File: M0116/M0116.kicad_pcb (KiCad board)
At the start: 2 copper layers, 38 x 17 mm, 2 parts, among them J2 Conn_01x04

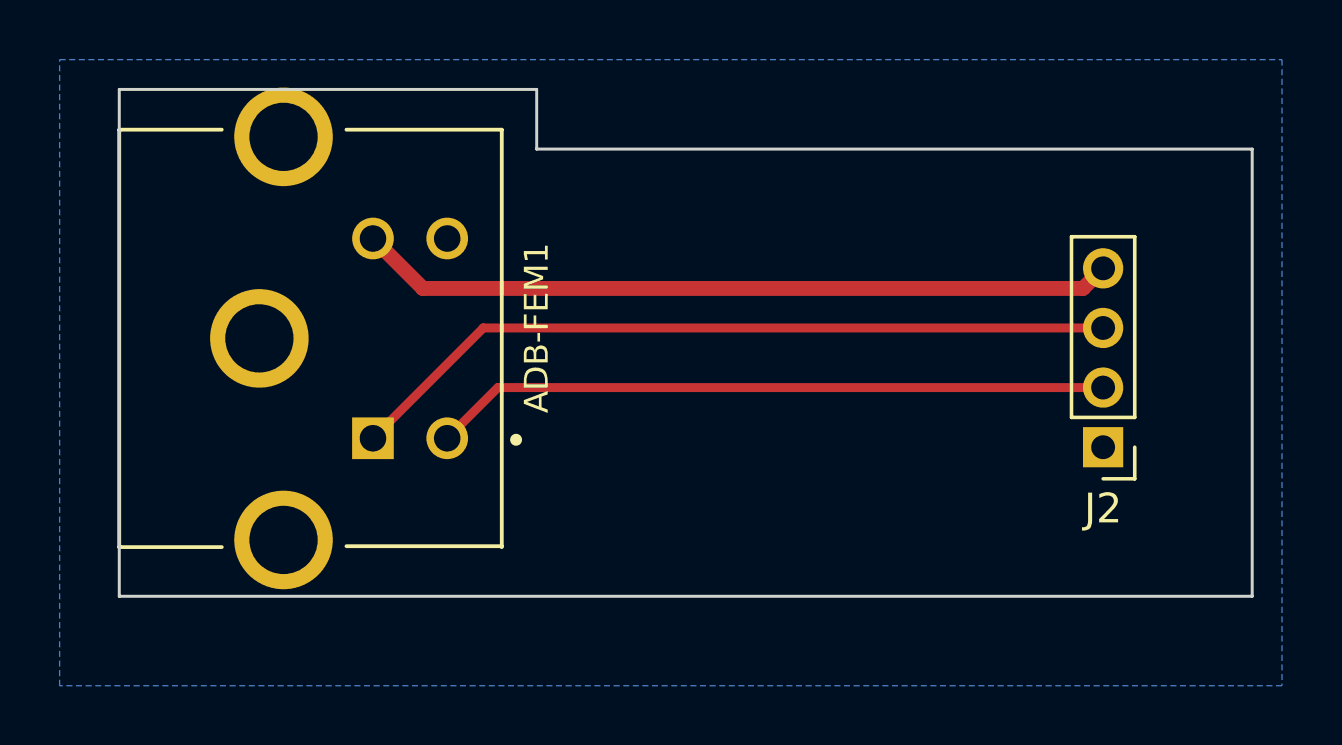
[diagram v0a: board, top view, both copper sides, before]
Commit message: added fabrication outputs
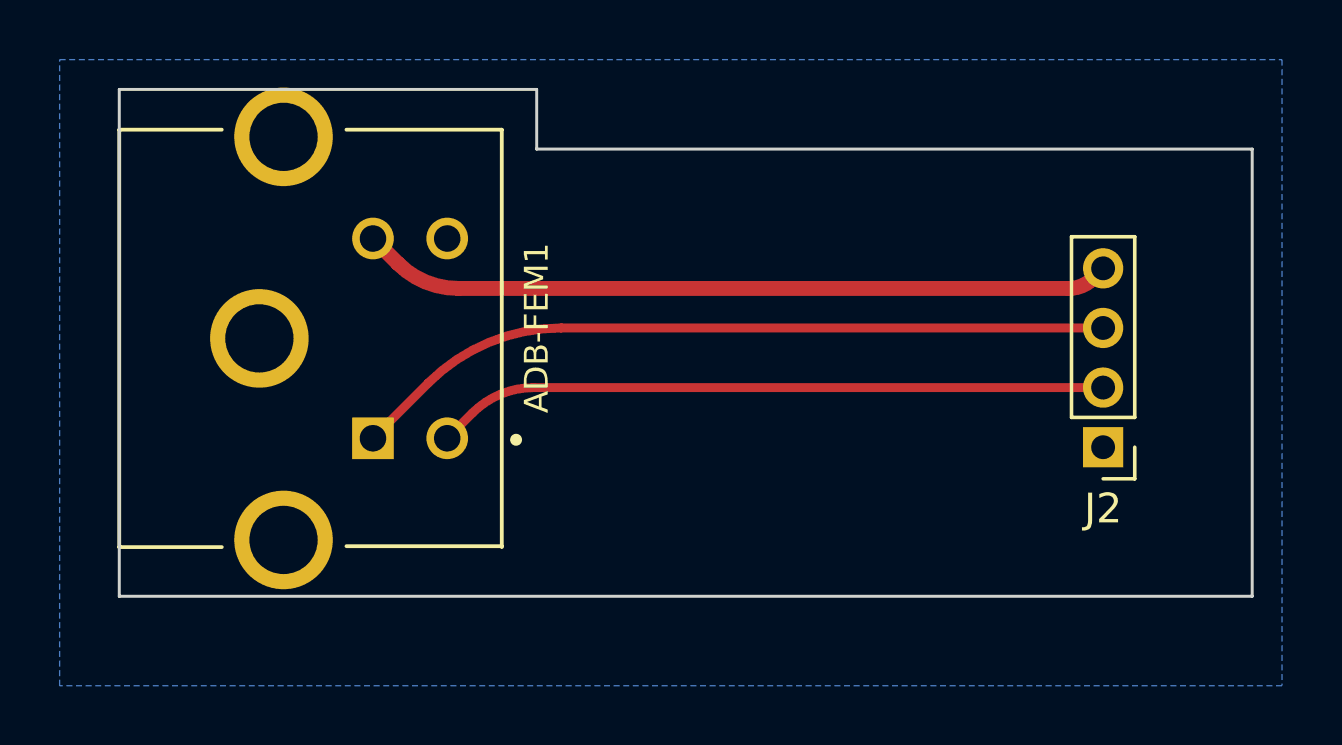
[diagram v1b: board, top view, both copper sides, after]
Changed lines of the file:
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@@
   (gr_line (start 114 102) (end 114 100)
     (stroke (width 0.1) (type default)) (layer "Edge.Cuts"))
-  (segment (start 133 108) (end 112.21 108) (width 0.3) (layer "F.Cu") (net 1))
-  (segment (start 112.21 108) (end 108.51 111.7) (width 0.3) (layer "F.Cu") (net 1))
-  (segment (start 112.7 110) (end 111 111.7) (width 0.3) (layer "F.Cu") (net 2))
-  (segment (start 133 110) (end 112.7 110) (width 0.3) (layer "F.Cu") (net 2))
-  (segment (start 133 106) (end 132.325 106.675) (width 0.5) (layer "F.Cu") (net 3))
-  (segment (start 110.185 106.675) (end 108.51 105) (width 0.5) (layer "F.Cu") (net 3))
-  (segment (start 132.325 106.675) (end 110.185 106.675) (width 0.5) (layer "F.Cu") (net 3))
+  (segment (start 114.826295 108) (end 133 108) (width 0.3) (layer "F.Cu") (net 1))
+  (segment (start 110.36 109.85) (end 108.51 111.7) (width 0.3) (layer "F.Cu") (net 1))
+  (arc (start 114.826295 108) (mid 112.409153 108.480799) (end 110.36 109.85) (width 0.3) (layer "F.Cu") (net 1))
+  (segment (start 111.85 110.85) (end 111 111.7) (width 0.3) (layer "F.Cu") (net 2))
+  (segment (start 113.902081 110) (end 133 110) (width 0.3) (layer "F.Cu") (net 2))
+  (arc (start 113.902081 110) (mid 112.791502 110.220907) (end 111.85 110.85) (width 0.3) (layer "F.Cu") (net 2))
+  (segment (start 132.6625 106.3375) (end 133 106) (width 0.5) (layer "F.Cu") (net 3))
+  (segment (start 109.3475 105.8375) (end 108.51 105) (width 0.5) (layer "F.Cu") (net 3))
+  (segment (start 111.369403 106.675) (end 131.847702 106.675) (width 0.5) (layer "F.Cu") (net 3))
+  (arc (start 132.6625 106.3375) (mid 132.288667 106.587286) (end 131.847702 106.675) (width 0.5) (layer "F.Cu") (net 3))
+  (arc (start 109.3475 105.8375) (mid 110.275157 106.45734) (end 111.369403 106.675) (width 0.5) (layer "F.Cu") (net 3))
+  (zone (net 2) (net_name "JST-D-") (layer "F.Cu") (name "$teardrop_padvia$") (hatch edge 0.5)
+    (priority 30004)
+    (attr (teardrop (type padvia)))
+    (connect_pads yes (clearance 0))
+    (min_thickness 0.0254) (filled_areas_thickness no)
+    (fill yes (thermal_gap 0.5) (thermal_bridge_width 0.5) (island_removal_mode 1) (island_area_min 10))
+    (polygon
+      (pts
+        (xy 131.65 109.85)
+        (xy 131.65 110.15)
+        (xy 132.741689 110.623619)
+        (xy 133.001 110)
+        (xy 132.741689 109.376381)
+      )
+    )
+  )
+  (zone (net 1) (net_name "JST-D+") (layer "F.Cu") (name "$teardrop_padvia$") (hatch edge 0.5)
+    (priority 30000)
+    (attr (teardrop (type padvia)))
+    (connect_pads yes (clearance 0))
+    (min_thickness 0.0254) (filled_areas_thickness no)
+    (fill yes (thermal_gap 0.5) (thermal_bridge_width 0.5) (island_removal_mode 1) (island_area_min 10))
+    (polygon
+      (pts
+        (xy 109.809333 110.612799)
+        (xy 109.597201 110.400667)
+        (xy 108.220465 111.001)
+        (xy 108.509293 111.700707)
+        (xy 109.208999 111.989535)
+      )
+    )
+  )
+  (zone (net 2) (net_name "JST-D-") (layer "F.Cu") (name "$teardrop_padvia$") (hatch edge 0.5)
+    (priority 30002)
+    (attr (teardrop (type padvia)))
+    (connect_pads yes (clearance 0))
+    (min_thickness 0.0254) (filled_areas_thickness no)
+    (fill yes (thermal_gap 0.5) (thermal_bridge_width 0.5) (island_removal_mode 1) (island_area_min 10))
+    (polygon
+      (pts
+        (xy 112.094601 110.817531)
+        (xy 111.882469 110.605399)
+        (xy 110.732504 111.054208)
+        (xy 110.999293 111.700707)
+        (xy 111.645792 111.967496)
+      )
+    )
+  )
+  (zone (net 3) (net_name "VBUS") (layer "F.Cu") (name "$teardrop_padvia$") (hatch edge 0.5)
+    (priority 30001)
+    (attr (teardrop (type padvia)))
+    (connect_pads yes (clearance 0))
+    (min_thickness 0.0254) (filled_areas_thickness no)
+    (fill yes (thermal_gap 0.5) (thermal_bridge_width 0.5) (island_removal_mode 1) (island_area_min 10))
+    (polygon
+      (pts
+        (xy 109.321758 106.165312)
+        (xy 109.675312 105.811758)
+        (xy 109.155792 104.732504)
+        (xy 108.509293 104.999293)
+        (xy 108.242504 105.645792)
+      )
+    )
+  )
+  (zone (net 1) (net_name "JST-D+") (layer "F.Cu") (name "$teardrop_padvia$") (hatch edge 0.5)
+    (priority 30003)
+    (attr (teardrop (type padvia)))
+    (connect_pads yes (clearance 0))
+    (min_thickness 0.0254) (filled_areas_thickness no)
+    (fill yes (thermal_gap 0.5) (thermal_bridge_width 0.5) (island_removal_mode 1) (island_area_min 10))
+    (polygon
+      (pts
+        (xy 131.65 107.85)
+        (xy 131.65 108.15)
+        (xy 132.741689 108.623619)
+        (xy 133.001 108)
+        (xy 132.741689 107.376381)
+      )
+    )
+  )
+  (zone (net 3) (net_name "VBUS") (layer "F.Cu") (name "$teardrop_padvia$") (hatch edge 0.5)
+    (priority 30005)
+    (attr (teardrop (type padvia)))
+    (connect_pads yes (clearance 0))
+    (min_thickness 0.0254) (filled_areas_thickness no)
+    (fill yes (thermal_gap 0.5) (thermal_bridge_width 0.5) (island_removal_mode 1) (island_area_min 10))
+    (polygon
+      (pts
+        (xy 131.929594 106.425)
+        (xy 131.929594 106.925)
+        (xy 133.258311 106.623619)
+        (xy 133.001 106)
+        (xy 132.376381 105.741689)
+      )
+    )
+  )
   (zone (net 4) (net_name "GND") (layer "B.Cu") (hatch edge 0.5)
     (connect_pads (clearance 0.5))
